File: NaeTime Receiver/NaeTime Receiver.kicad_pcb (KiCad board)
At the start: 2 copper layers, 135 x 140 mm, 22 parts, among them U15 RX5808_Breakout, U16 RX5808_Breakout, U17 RX5808_Breakout, U18 RX5808_Breakout, U19 RX5808_Breakout, U20 RX5808_Breakout, U21 RX5808_Breakout, U22 RX5808_Breakout

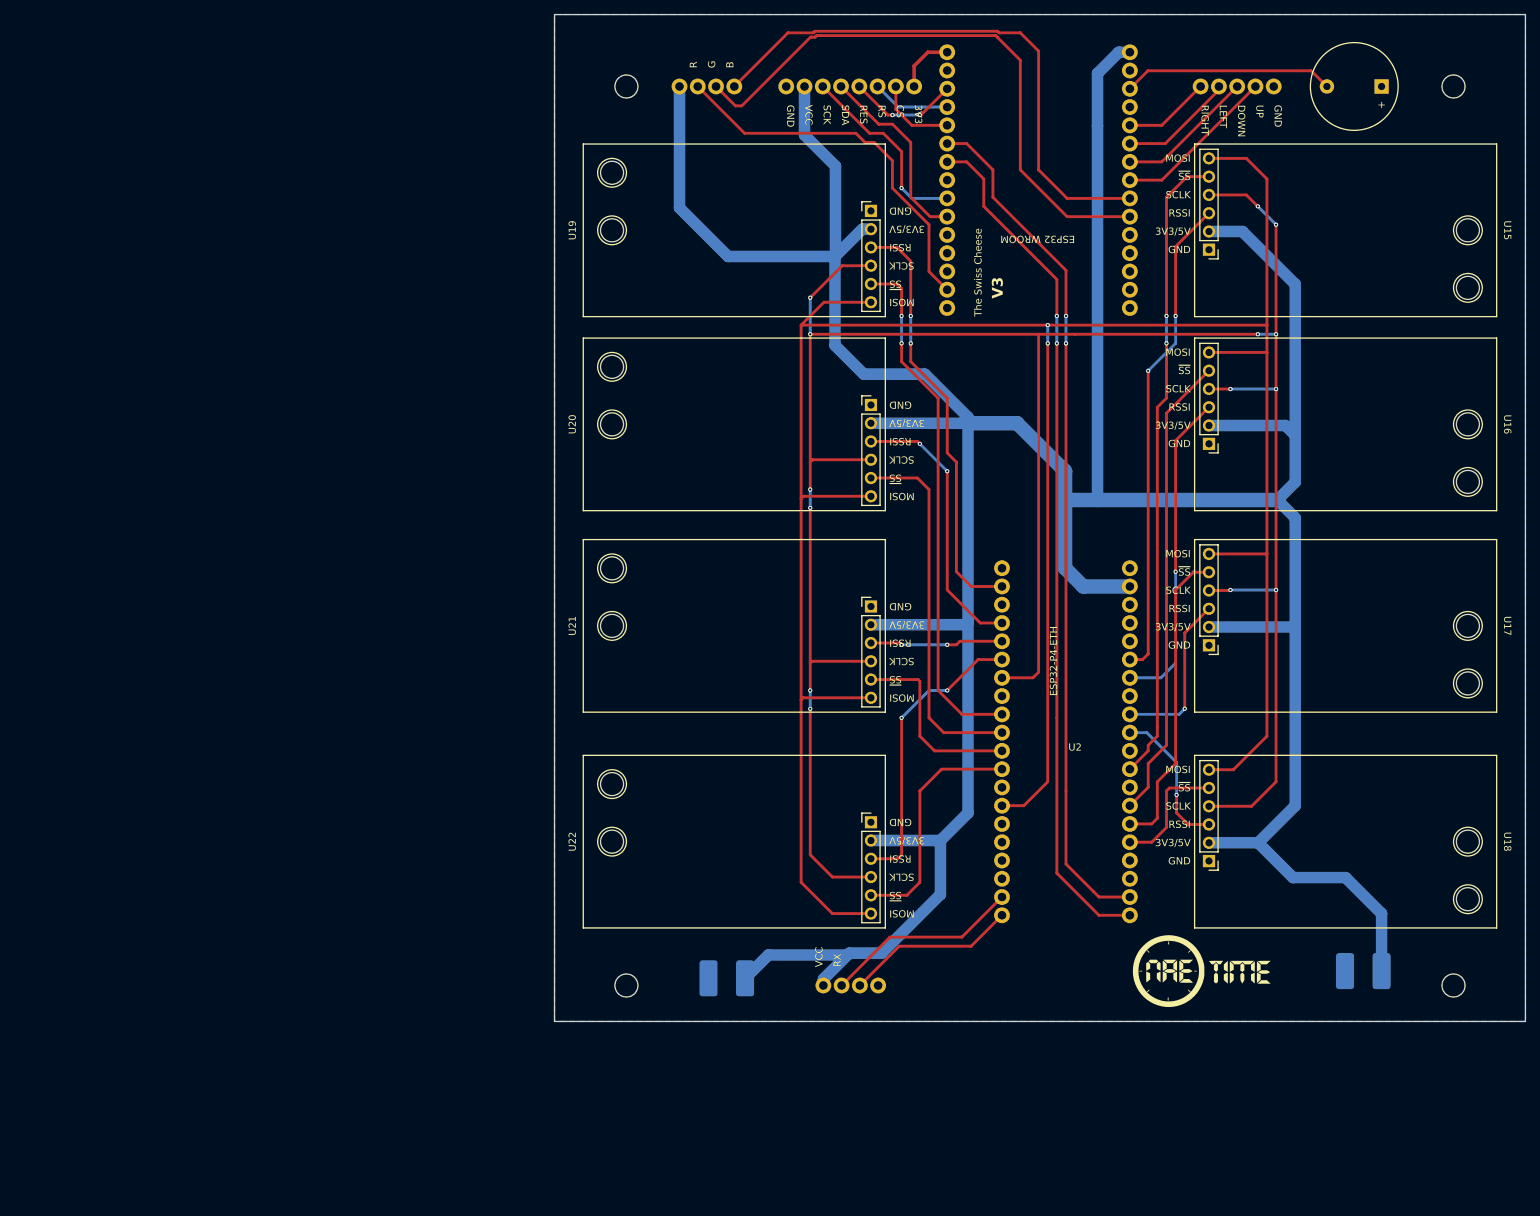
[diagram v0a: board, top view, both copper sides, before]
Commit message: Receiver pcb
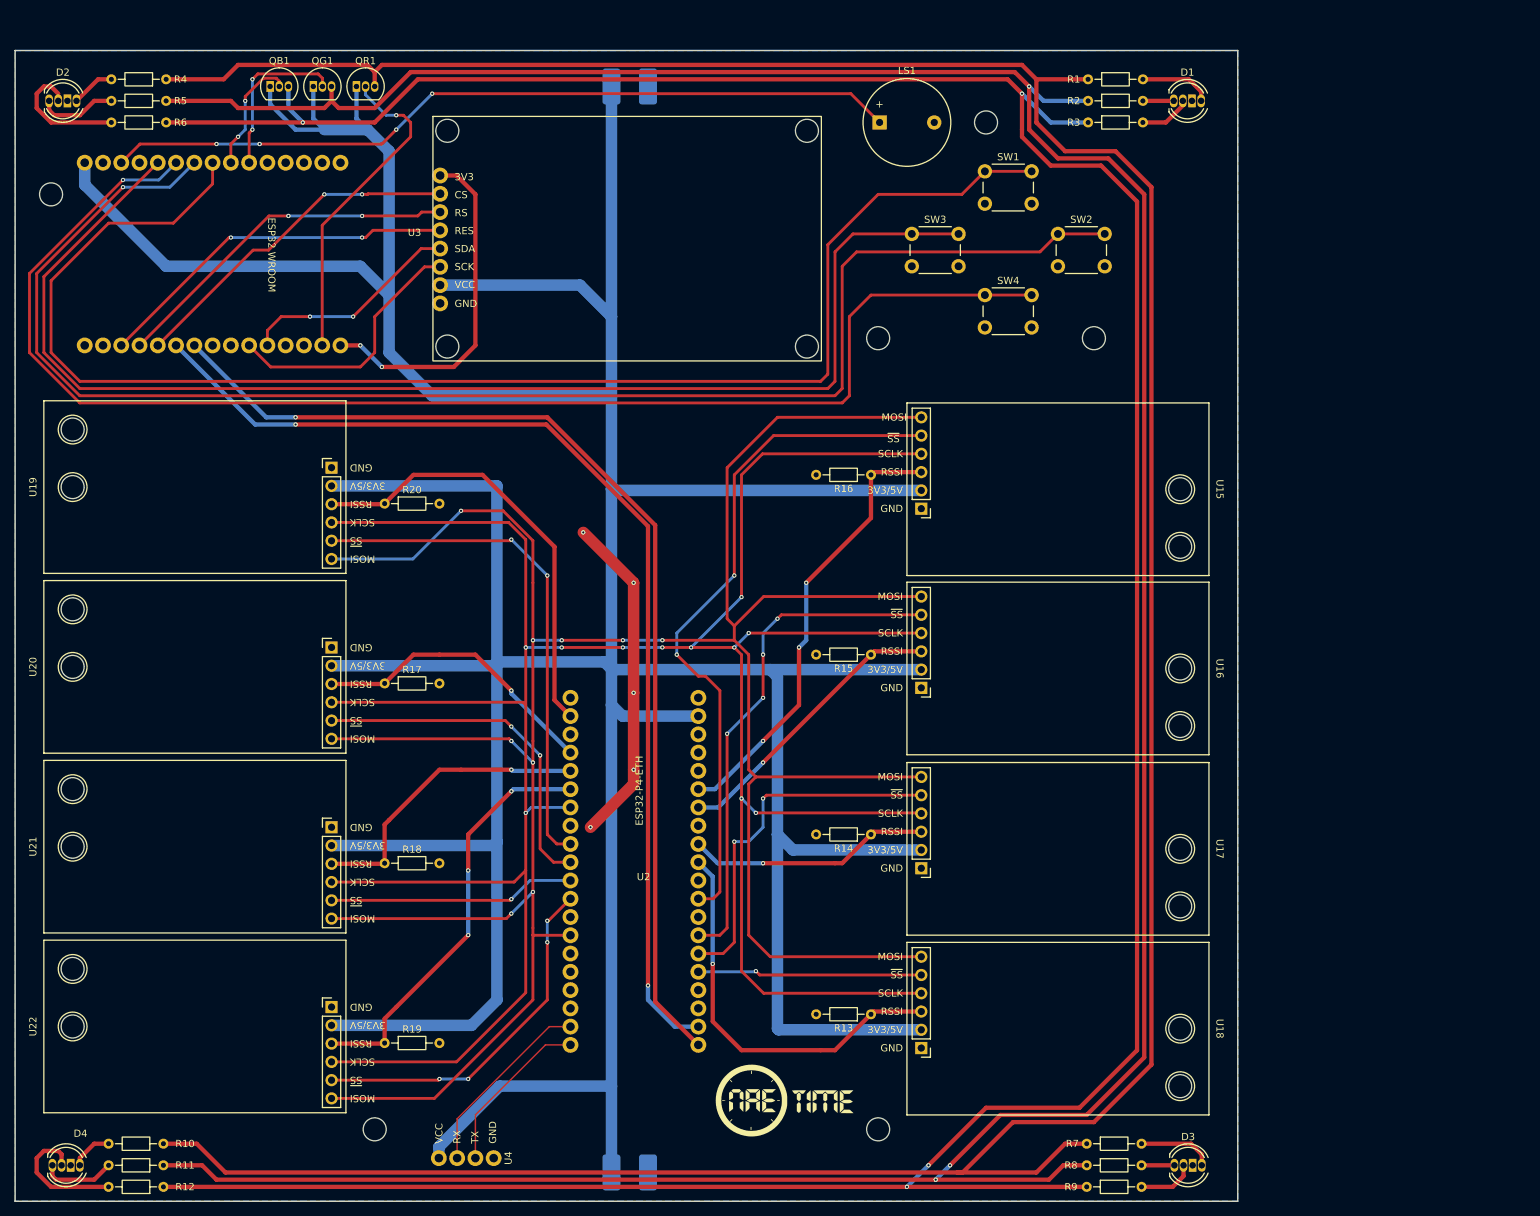
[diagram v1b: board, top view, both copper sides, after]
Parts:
- removed the REF** at (100.0, 20.0)
- removed the REF** at (100.0, 145.0)
- removed the REF** at (215.0, 145.0)
- removed the REF** at (215.0, 20.0)
- removed U5: ~, NaeTimeComponentLibrary:RGB LED Header
- removed U6: ~, NaeTimeComponentLibrary:DPad Pin Header
- added D1: CLV1L-FKB, NaeTimeComponentLibrary:LED_D5.0mm-4_RGB GBCR, F.Cu at (176.1, 22.0)
- added D2: CLV1L-FKB, NaeTimeComponentLibrary:LED_D5.0mm-4_RGB GBCR, F.Cu at (19.7, 22.0)
- added D3: CLV1L-FKB, NaeTimeComponentLibrary:LED_D5.0mm-4_RGB GBCR, F.Cu at (176.2, 170.0)
- added D4: CLV1L-FKB, NaeTimeComponentLibrary:LED_D5.0mm-4_RGB GBCR, F.Cu at (20.2, 170.0)
- added QB1: BS170, Package_TO_SOT_THT:TO-92_Inline, F.Cu at (50.5, 20.0)
- added QG1: BS170, Package_TO_SOT_THT:TO-92_Inline, F.Cu at (56.5, 20.0)
- added QR1: BS170, Package_TO_SOT_THT:TO-92_Inline, F.Cu at (62.5, 20.0)
- added R1: R2, Resistor_THT:R_Axial_DIN0204_L3.6mm_D1.6mm_P7.62mm_Horizontal, F.Cu at (164.2, 19.0)
- added R10: R2, Resistor_THT:R_Axial_DIN0204_L3.6mm_D1.6mm_P7.62mm_Horizontal, F.Cu at (35.6, 167.0)
- added R11: R3, Resistor_THT:R_Axial_DIN0204_L3.6mm_D1.6mm_P7.62mm_Horizontal, F.Cu at (35.6, 170.0)
- added R12: R4, Resistor_THT:R_Axial_DIN0204_L3.6mm_D1.6mm_P7.62mm_Horizontal, F.Cu at (35.6, 173.0)
- added R13: R1, Resistor_THT:R_Axial_DIN0204_L3.6mm_D1.6mm_P7.62mm_Horizontal, F.Cu at (134.0, 149.0)
- added R14: R1, Resistor_THT:R_Axial_DIN0204_L3.6mm_D1.6mm_P7.62mm_Horizontal, F.Cu at (134.0, 124.0)
- added R15: R1, Resistor_THT:R_Axial_DIN0204_L3.6mm_D1.6mm_P7.62mm_Horizontal, F.Cu at (134.0, 99.0)
- added R16: R1, Resistor_THT:R_Axial_DIN0204_L3.6mm_D1.6mm_P7.62mm_Horizontal, F.Cu at (134.0, 74.0)
- added R17: R1, Resistor_THT:R_Axial_DIN0204_L3.6mm_D1.6mm_P7.62mm_Horizontal, F.Cu at (66.4, 103.0)
- added R18: R1, Resistor_THT:R_Axial_DIN0204_L3.6mm_D1.6mm_P7.62mm_Horizontal, F.Cu at (66.4, 128.0)
- added R19: R1, Resistor_THT:R_Axial_DIN0204_L3.6mm_D1.6mm_P7.62mm_Horizontal, F.Cu at (66.4, 153.0)
- added R2: R3, Resistor_THT:R_Axial_DIN0204_L3.6mm_D1.6mm_P7.62mm_Horizontal, F.Cu at (164.2, 22.0)
- added R20: R1, Resistor_THT:R_Axial_DIN0204_L3.6mm_D1.6mm_P7.62mm_Horizontal, F.Cu at (66.4, 78.0)
- added R3: R4, Resistor_THT:R_Axial_DIN0204_L3.6mm_D1.6mm_P7.62mm_Horizontal, F.Cu at (164.2, 25.0)
- added R4: R2, Resistor_THT:R_Axial_DIN0204_L3.6mm_D1.6mm_P7.62mm_Horizontal, F.Cu at (36.0, 19.0)
- added R5: R3, Resistor_THT:R_Axial_DIN0204_L3.6mm_D1.6mm_P7.62mm_Horizontal, F.Cu at (36.0, 22.0)
- added R6: R4, Resistor_THT:R_Axial_DIN0204_L3.6mm_D1.6mm_P7.62mm_Horizontal, F.Cu at (36.0, 25.0)
- added R7: R2, Resistor_THT:R_Axial_DIN0204_L3.6mm_D1.6mm_P7.62mm_Horizontal, F.Cu at (164.0, 167.0)
- added R8: R3, Resistor_THT:R_Axial_DIN0204_L3.6mm_D1.6mm_P7.62mm_Horizontal, F.Cu at (164.0, 170.0)
- added R9: R4, Resistor_THT:R_Axial_DIN0204_L3.6mm_D1.6mm_P7.62mm_Horizontal, F.Cu at (164.0, 173.0)
- added REF**: MountingHole_3.2mm_M3, MountingHole:MountingHole_3.2mm_M3, F.Cu at (135.0, 55.0)
- added REF**: MountingHole_3.2mm_M3, MountingHole:MountingHole_3.2mm_M3, F.Cu at (150.0, 25.0)
- added REF**: MountingHole_3.2mm_M3, MountingHole:MountingHole_3.2mm_M3, F.Cu at (135.0, 165.0)
- added REF**: MountingHole_3.2mm_M3, MountingHole:MountingHole_3.2mm_M3, F.Cu at (165.0, 55.0)
- added REF**: MountingHole_3.2mm_M3, MountingHole:MountingHole_3.2mm_M3, F.Cu at (20.0, 35.0)
- added REF**: MountingHole_3.2mm_M3, MountingHole:MountingHole_3.2mm_M3, F.Cu at (65.0, 165.0)
- added SW1: SW_Push, Button_Switch_THT:SW_PUSH_6mm_H5mm, F.Cu at (149.8, 31.8)
- added SW2: SW_Push, Button_Switch_THT:SW_PUSH_6mm_H5mm, F.Cu at (160.0, 40.5)
- added SW3: SW_Push, Button_Switch_THT:SW_PUSH_6mm_H5mm, F.Cu at (139.7, 40.5)
- added SW4: SW_Push, Button_Switch_THT:SW_PUSH_6mm_H5mm, F.Cu at (149.8, 49.0)
- moved U7 124.7 mm to (100.5, 20.0), turned to 90 degrees
- moved U1 115.3 mm to (42.5, 43.3), turned to -90 degrees
- moved U8 105.8 mm to (100.5, 171.0), turned to 90 degrees
- moved U19 83.1 mm to (40.0, 75.7)
- moved U20 82.2 mm to (40.0, 100.7)
- moved U21 81.0 mm to (40.0, 125.7)
- moved U22 79.3 mm to (40.0, 150.7)
- moved LS1 70.0 mm to (135.2, 25.0), turned to 0 degrees
- moved U2 62.6 mm to (92.2, 130.4)
- moved G*** 60.7 mm to (122.0, 161.0)
- moved U3 60.4 mm to (73.1, 40.6), turned to 0 degrees
- moved U4 58.6 mm to (79.0, 169.0)
- moved U15 53.8 mm to (160.0, 76.0)
- moved U16 52.5 mm to (160.0, 100.9)
- moved U17 50.6 mm to (160.0, 126.0)
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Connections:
- LS1 pad 1: GND -> Net-(LS1-Pad1)
- LS1 pad 2: Net-(LS1-Pad2) -> GND
- U1 pad 13: Net-(LS1-Pad2) -> Net-(LS1-Pad1)
- U1 pad 16: unconnected-(U1-23/MOSI-Pad16) -> Net-(U1-23/MOSI)
- U1 pad 17: Net-(U1-22/SCL) -> RED SWITCH
- U1 pad 20: unconnected-(U1-21/MISO-Pad20) -> Net-(U1-21/MISO)
- U1 pad 21: Net-(U1-19/MISO) -> Net-(U1-19/SCK)
- U1 pad 22: Net-(U1-18/SCK) -> unconnected-(U1-18-Pad22)
- U1 pad 6: Net-(U1-32) -> GREEN SWITCH
- U1 pad 7: Net-(U1-33) -> BLUE SWITCH
- U3 pad 3: Net-(U1-18/SCK) -> Net-(U1-19/SCK)
- U3 pad 4: Net-(U1-19/MISO) -> Net-(U1-21/MISO)
- U3 pad 8: +3.3V -> Net-(U1-23/MOSI)
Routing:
- net BLUE: track 0.00 -> 451.0 mm, vias 0 -> 4
- net GREEN: track 0.00 -> 447.0 mm, vias 0 -> 3
- net RED: track 0.00 -> 445.3 mm
- net Net-(U1-26): track 19.3 -> 209.6 mm, vias 0 -> 1
- net +5V: track 542.6 -> 723.8 mm
- net Net-(U1-25): track 22.9 -> 201.6 mm
- net Net-(U1-27): track 16.0 -> 192.7 mm, vias 0 -> 1
- net Net-(U1-14): track 12.1 -> 181.7 mm
- net Net-(LS1-Pad1): track 0.00 -> 111.1 mm, vias 0 -> 4
- net Net-(U1-32): track 82.1 -> 0.00 mm
- net Net-(U1-33): track 77.5 -> 0.00 mm
- net Net-(U1-22/SCL): track 52.4 -> 0.00 mm
- net Net-(U1-23/MOSI): track 0.00 -> 48.2 mm, vias 0 -> 2
- net GND: track 0.00 -> 46.4 mm, vias 0 -> 5
- net RED SWITCH: track 0.00 -> 45.1 mm, vias 0 -> 1
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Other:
- board size 135 x 140 mm -> 170 x 160 mm
- board text removed: "5V"
- board text removed: "The Swiss Cheese"
- board text removed: "V3"
